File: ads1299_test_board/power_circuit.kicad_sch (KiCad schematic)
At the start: 16 parts, among them J1 Conn_01x02, SW1 SW_Push, U6 AP2112K-3.3

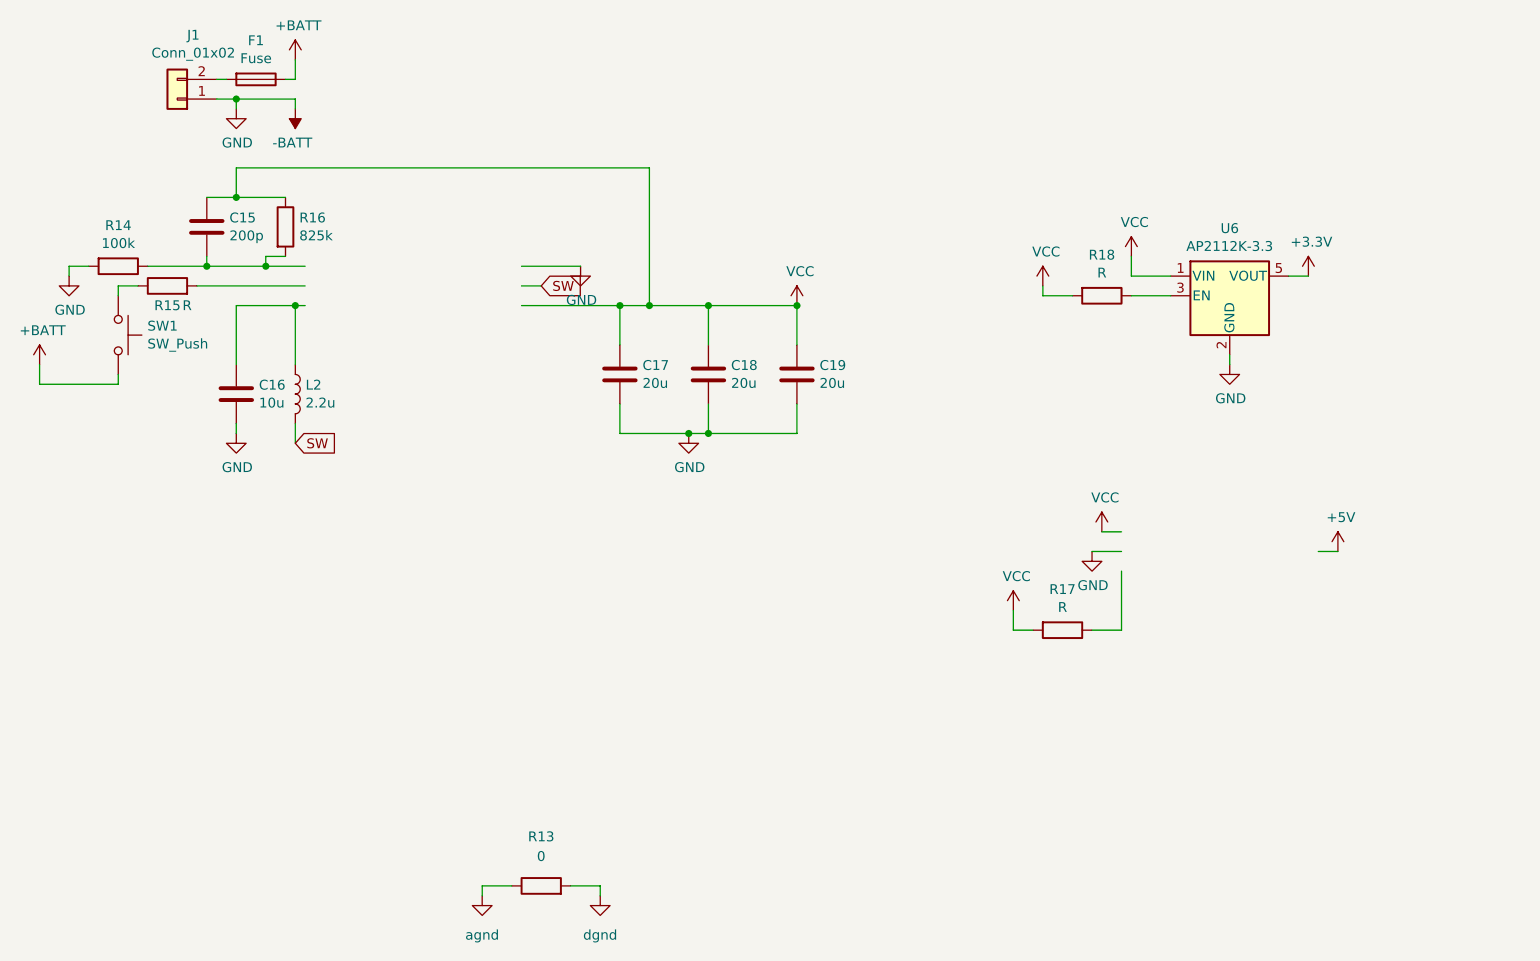
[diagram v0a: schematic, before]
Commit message: charger circuit
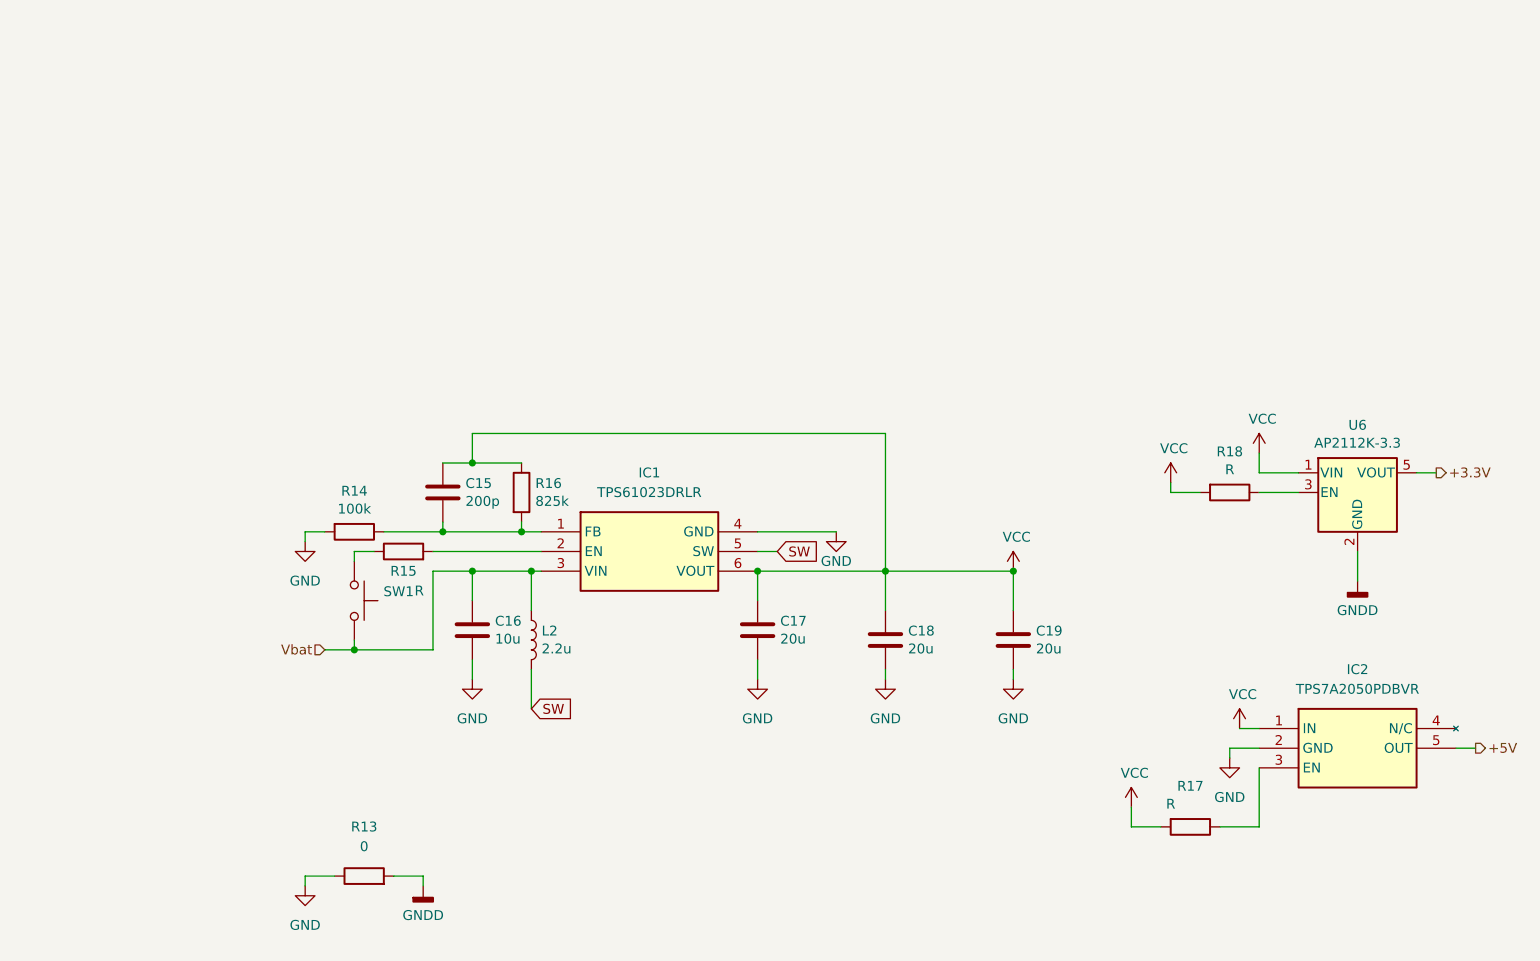
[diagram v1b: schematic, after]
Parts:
- removed F1: Fuse, symbol Device:Fuse
- removed J1: Conn_01x02, symbol Connector_Generic:Conn_01x02
- added IC1: TPS61023DRLR, SOTFL50P160X60-6N, symbol TPS61023DRLR:TPS61023DRLR
- added IC2: TPS7A2050PDBVR, SOT95P280X145-5N, symbol TPS7A2050PDBVR:TPS7A2050PDBVR
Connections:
- net +BATT is gone; now on net Vbat: SW1.2
- net agnd is gone; now on net GND: R13.1
- net +5V: now also IC2.5 (OUT)
- net SW: now also IC1.5 (SW)
- net VCC: now also IC1.6 (VOUT), IC2.1 (IN)
- net at R15.2: now also IC1.2 (EN)
- net at R17.1: now also IC2.3 (EN)
- net at C15.2, R14.1, R16.2: now also IC1.1 (FB)
- net Vbat: now reaches C16.1, L2.1
- net Vbat: now also IC1.3 (VIN)
- net -BATT renamed GND
- net GND: now also IC1.4 (GND), IC2.2 (GND); no longer U6.2 (GND)
- net dgnd renamed GNDD
- net GNDD: now also U6.2 (GND)
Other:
- moved on the sheet: C15, C16, C17, C18, C19, L2, R13, R14, R15, R16, R17, R18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
